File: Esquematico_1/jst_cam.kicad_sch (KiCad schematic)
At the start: 19 parts, among them J1 Screw_Terminal_01x04, J2 Screw_Terminal_01x03, J3 Screw_Terminal_01x06, J4 Screw_Terminal_01x08, J5 USB_C_Receptacle_USB2.0_14P, J6 Screw_Terminal_01x05, U5 USBLC6-2SC6

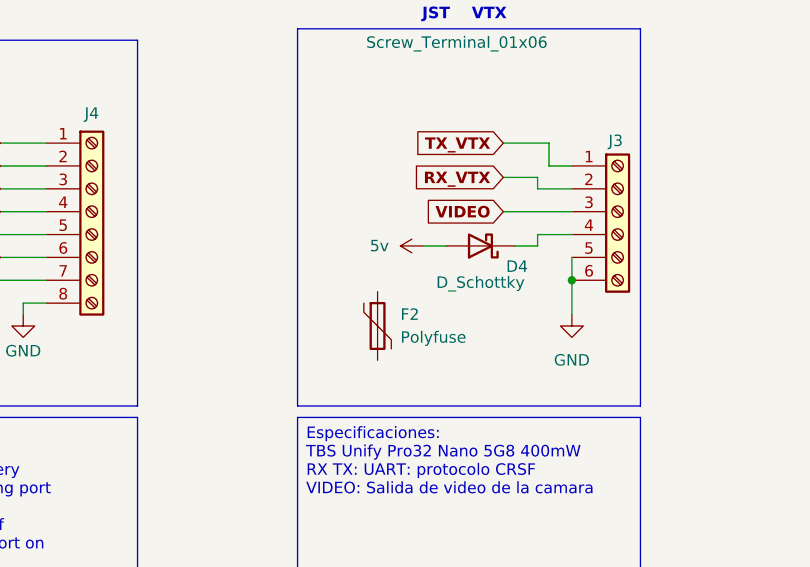
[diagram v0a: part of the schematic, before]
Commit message: Footprints
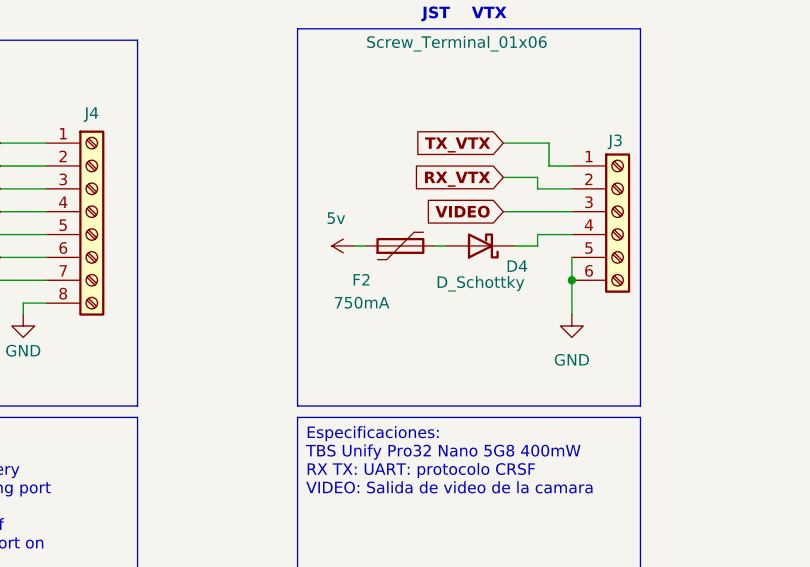
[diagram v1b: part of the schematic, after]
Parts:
- F2: value Polyfuse -> 750mA; footprint (none) -> Capacitor_SMD:C_0805_2012Metric_Pad1.18x1.45mm_HandSolder
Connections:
- net 5v: now also F2.1; no longer D4.2 (A)
- net at F2.2: now also D4.2 (A)
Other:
- moved on the sheet: F2
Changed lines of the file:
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@@
+	(wire
+		(pts
+			(xy 102.87 46.99) (xy 104.14 46.99)
+		)
+		(stroke
+			(width 0)
+			(type default)
+		)
+	)
 	(wire
 		(pts
@@
 	(wire
 		(pts
+			(xy 111.76 46.99) (xy 113.03 46.99)
+		)
+		(stroke
+			(width 0)
+			(type default)
+		)
+	)
+	(wire
+		(pts
 			(xy 144.78 128.27) (xy 154.94 128.27)
 		)
@@
 		(pts
 			(xy 119.38 39.37) (xy 123.19 39.37)
-		)
-		(stroke
-			(width 0)
-			(type default)
-		)
-	)
-	(wire
-		(pts
-			(xy 113.03 46.99) (xy 110.49 46.99)
 		)
 		(stroke
@@
 	(symbol
 		(lib_id "Device:Polyfuse")
-		(at 105.41 55.88 0)
+		(at 107.95 46.99 90)
 		(unit 1)
 		(exclude_from_sim no)
@@
 		(on_board yes)
 		(dnp no)
-		(fields_autoplaced yes)
 		(property "Reference" "F2"
-			(at 107.95 54.6099 0)
-			(effects
-				(font
-					(size 1.27 1.27)
-				)
-				(justify left)
-			)
-		)
-		(property "Value" "Polyfuse"
-			(at 107.95 57.1499 0)
-			(effects
-				(font
-					(size 1.27 1.27)
-				)
-				(justify left)
-			)
-		)
-		(property "Footprint" ""
-			(at 106.68 60.96 0)
+			(at 103.632 50.8 90)
+			(effects
+				(font
+					(size 1.27 1.27)
+				)
+			)
+		)
+		(property "Value" "750mA"
+			(at 103.632 53.34 90)
+			(effects
+				(font
+					(size 1.27 1.27)
+				)
+			)
+		)
+		(property "Footprint" "Capacitor_SMD:C_0805_2012Metric_Pad1.18x1.45mm_HandSolder"
+			(at 113.03 45.72 0)
 			(effects
 				(font
@@
 		)
 		(property "Datasheet" "~"
-			(at 105.41 55.88 0)
+			(at 107.95 46.99 0)
 			(effects
 				(font
@@
 		)
 		(property "Description" "Resettable fuse, polymeric positive temperature coefficient"
-			(at 105.41 55.88 0)
+			(at 107.95 46.99 0)
 			(effects
 				(font
@@
 	(symbol
 		(lib_id "power:+3.3V")
-		(at 110.49 46.99 90)
+		(at 102.87 46.99 90)
 		(unit 1)
 		(exclude_from_sim no)
@@
 		(on_board yes)
 		(dnp no)
-		(fields_autoplaced yes)
 		(property "Reference" "#PWR046"
-			(at 114.3 46.99 0)
+			(at 106.68 46.99 0)
 			(effects
 				(font
@@
 		)
 		(property "Value" "5v"
-			(at 106.68 46.9899 90)
+			(at 101.854 43.942 90)
 			(effects
 				(font
@@
 		)
 		(property "Footprint" ""
-			(at 110.49 46.99 0)
+			(at 102.87 46.99 0)
 			(effects
 				(font
@@
 		)
 		(property "Datasheet" ""
-			(at 110.49 46.99 0)
+			(at 102.87 46.99 0)
 			(effects
 				(font
@@
 		)
 		(property "Description" "Power symbol creates a global label with name \"+3.3V\""
-			(at 110.49 46.99 0)
-			(effects
-				(font
+			(at 102.87 46.99 0)
+			(effects
+				(font

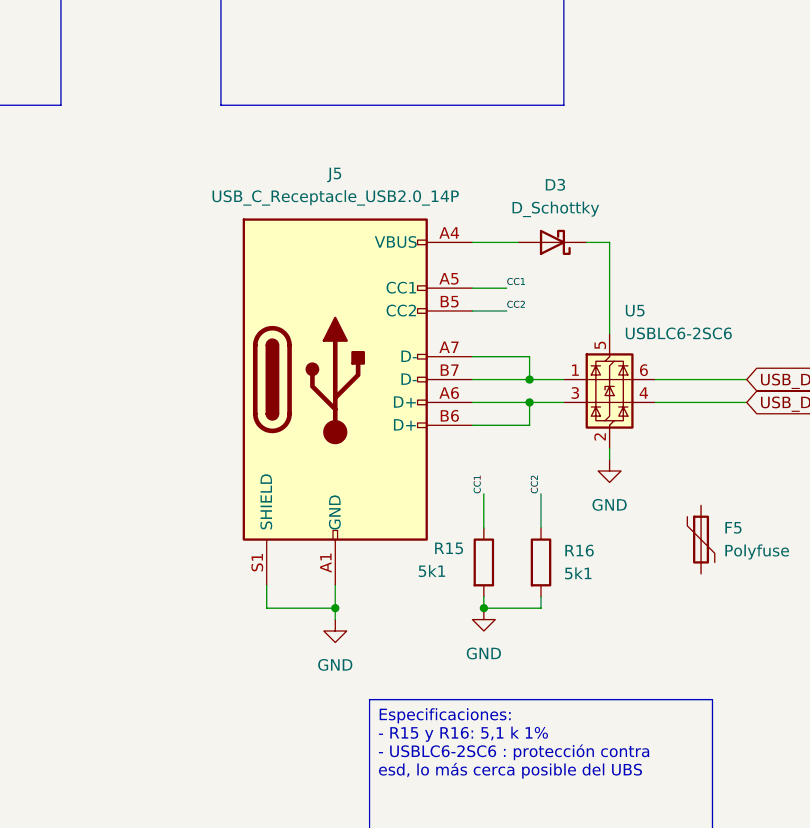
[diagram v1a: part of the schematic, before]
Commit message: USB 16 Pin
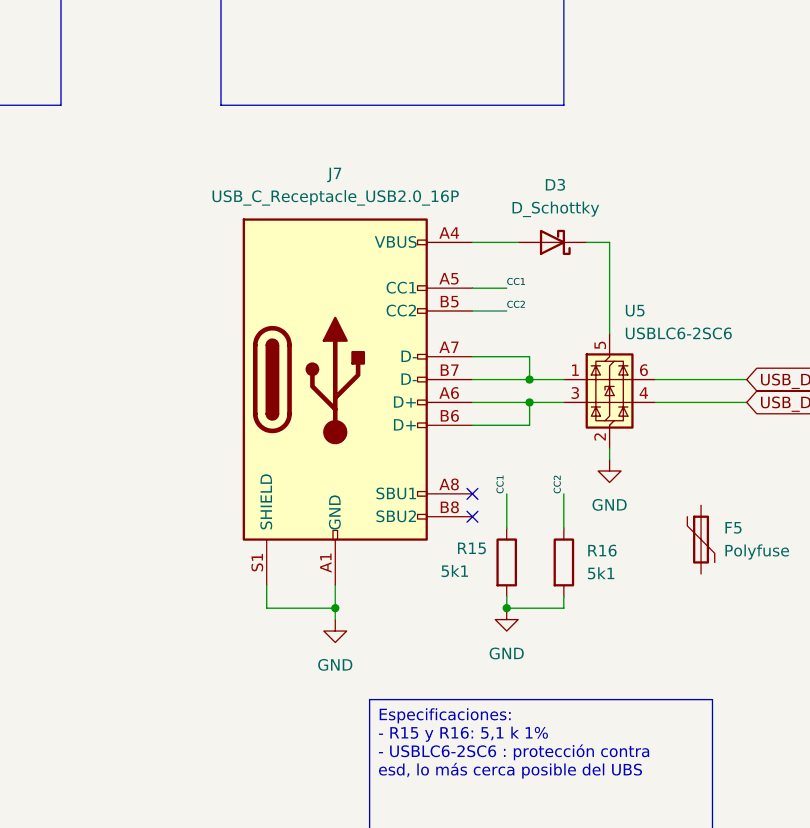
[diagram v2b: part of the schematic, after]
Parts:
- removed J5: USB_C_Receptacle_USB2.0_14P, symbol Connector:USB_C_Receptacle_USB2.0_14P
- added J7: USB_C_Receptacle_USB2.0_16P, symbol Connector:USB_C_Receptacle_USB2.0_16P
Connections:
- net CC1: now also J7.A5 (CC1)
- net CC2: now also J7.B5 (CC2)
- net GND: now also J7.A1 (GND), J7.A12 (GND), J7.B1 (GND), J7.B12 (GND), J7.S1 (SHIELD)
- net at D3.2 (A): now also J7.A4 (VBUS), J7.A9 (VBUS), J7.B4 (VBUS), J7.B9 (VBUS)
- net at U5.3 (I/O2): now also J7.A6 (D+), J7.B6 (D+)
- net at U5.1 (I/O1): now also J7.A7 (D-), J7.B7 (D-)
- no-connect marks 0 -> 2
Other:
- moved on the sheet: R15, R16
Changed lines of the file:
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@@
 	)
 	(junction
-		(at 125.73 153.67)
+		(at 128.27 153.67)
 		(diameter 0)
 		(color 0 0 0 0)
@@
 		(color 0 0 0 0)
 	)
+	(no_connect
+		(at 124.46 143.51)
+	)
+	(no_connect
+		(at 124.46 140.97)
+	)
 	(wire
 		(pts
@@
 	(wire
 		(pts
-			(xy 125.73 140.97) (xy 125.73 144.78)
+			(xy 128.27 140.97) (xy 128.27 144.78)
 		)
 		(stroke
@@
 	(wire
 		(pts
-			(xy 132.08 152.4) (xy 132.08 153.67)
+			(xy 134.62 152.4) (xy 134.62 153.67)
 		)
 		(stroke
@@
 	(wire
 		(pts
-			(xy 132.08 140.97) (xy 132.08 144.78)
+			(xy 134.62 140.97) (xy 134.62 144.78)
 		)
 		(stroke
@@
 	(wire
 		(pts
-			(xy 125.73 152.4) (xy 125.73 153.67)
+			(xy 128.27 152.4) (xy 128.27 153.67)
 		)
 		(stroke
@@
 	(wire
 		(pts
-			(xy 125.73 153.67) (xy 132.08 153.67)
+			(xy 128.27 153.67) (xy 134.62 153.67)
 		)
 		(stroke
@@
 	)
 	(label "CC1"
-		(at 125.73 140.97 90)
+		(at 128.27 140.97 90)
 		(effects
 			(font
@@
 	)
 	(label "CC2"
-		(at 132.08 140.97 90)
+		(at 134.62 140.97 90)
 		(effects
 			(font
@@
 	)
 	(symbol
-		(lib_id "Connector:USB_C_Receptacle_USB2.0_14P")
-		(at 109.22 128.27 0)
-		(unit 1)
-		(exclude_from_sim no)
-		(in_bom yes)
-		(on_board yes)
-		(dnp no)
-		(property "Reference" "J5"
-			(at 109.22 105.41 0)
-			(effects
-				(font
-					(size 1.27 1.27)
-				)
-			)
-		)
-		(property "Value" "USB_C_Receptacle_USB2.0_14P"
-			(at 109.22 107.95 0)
-			(effects
-				(font
-					(size 1.27 1.27)
-				)
-			)
-		)
-		(property "Footprint" ""
-			(at 113.03 128.27 0)
-			(effects
-				(font
-					(size 1.27 1.27)
-				)
-				(hide yes)
-			)
-		)
-		(property "Datasheet" "https://www.usb.org/sites/default/files/documents/usb_type-c.zip"
-			(at 113.03 128.27 0)
-			(effects
-				(font
-					(size 1.27 1.27)
-				)
-				(hide yes)
-			)
-		)
-		(property "Description" "USB 2.0-only 14P Type-C Receptacle connector"
-			(at 109.22 128.27 0)
-			(effects
-				(font
-					(size 1.27 1.27)
-				)
-				(hide yes)
-			)
-		)
-		(pin "B7"
-		)
-		(pin "B5"
-		)
-		(pin "B6"
-		)
-		(pin "A6"
-		)
-		(pin "B4"
-		)
-		(pin "A7"
-		)
-		(pin "S1"
-		)
-		(pin "B9"
-		)
-		(pin "A5"
-		)
-		(pin "A1"
-		)
-		(pin "A12"
-		)
-		(pin "B1"
-		)
-		(pin "B12"
-		)
-		(pin "A4"
-		)
-		(pin "A9"
-		)
-		(instances
-			(project "Esquematico_1"
-				(path "/de2d80c1-c21c-478d-b724-17659b714c38/457e76de-adfe-4ec5-a818-c5970caa89a7"
-					(reference "J5")
-					(unit 1)
-				)
-			)
-		)
-	)
-	(symbol
 		(lib_id "power:GND")
 		(at 66.04 54.61 0)
@@
 	)
 	(symbol
+		(lib_id "Connector:USB_C_Receptacle_USB2.0_16P")
+		(at 109.22 128.27 0)
+		(unit 1)
+		(exclude_from_sim no)
+		(in_bom yes)
+		(on_board yes)
+		(dnp no)
+		(fields_autoplaced yes)
+		(property "Reference" "J7"
+			(at 109.22 105.41 0)
+			(effects
+				(font
+					(size 1.27 1.27)
+				)
+			)
+		)
+		(property "Value" "USB_C_Receptacle_USB2.0_16P"
+			(at 109.22 107.95 0)
+			(effects
+				(font
+					(size 1.27 1.27)
+				)
+			)
+		)
+		(property "Footprint" ""
+			(at 113.03 128.27 0)
+			(effects
+				(font
+					(size 1.27 1.27)
+				)
+				(hide yes)
+			)
+		)
+		(property "Datasheet" "https://www.usb.org/sites/default/files/documents/usb_type-c.zip"
+			(at 113.03 128.27 0)
+			(effects
+				(font
+					(size 1.27 1.27)
+				)
+				(hide yes)
+			)
+		)
+		(property "Description" "USB 2.0-only 16P Type-C Receptacle connector"
+			(at 109.22 128.27 0)
+			(effects
+				(font
+					(size 1.27 1.27)
+				)
+				(hide yes)
+			)
+		)
+		(pin "B6"
+		)
+		(pin "B4"
+		)
+		(pin "A7"
+		)
+		(pin "A5"
+		)
+		(pin "A1"
+		)
+		(pin "A12"
+		)
+		(pin "A9"
+		)
+		(pin "S1"
+		)
+		(pin "A4"
+		)
+		(pin "B12"
+		)
+		(pin "B1"
+		)
+		(pin "B7"
+		)
+		(pin "A6"
+		)
+		(pin "B9"
+		)
+		(pin "B8"
+		)
+		(pin "B5"
+		)
+		(pin "A8"
+		)
+		(instances
+			(project ""
+				(path "/de2d80c1-c21c-478d-b724-17659b714c38/457e76de-adfe-4ec5-a818-c5970caa89a7"
+					(reference "J7")
+					(unit 1)
+				)
+			)
+		)
+	)
+	(symbol
 		(lib_id "Device:D_Schottky")
 		(at 133.35 113.03 180)
@@
 	(symbol
 		(lib_id "Device:R")
-		(at 132.08 148.59 0)
+		(at 134.62 148.59 0)
 		(unit 1)
 		(exclude_from_sim no)
@@
 		(fields_autoplaced yes)
 		(property "Reference" "R16"
-			(at 134.62 147.3199 0)
+			(at 137.16 147.3199 0)
 			(effects
 				(font
@@
 		)
 		(property "Value" "5k1"
-			(at 134.62 149.8599 0)
+			(at 137.16 149.8599 0)
 			(effects
 				(font
@@
 		)
 		(property "Footprint" "Resistor_SMD:R_0805_2012Metric_Pad1.20x1.40mm_HandSolder"
-			(at 130.302 148.59 90)
+			(at 132.842 148.59 90)
 			(effects
 				(font
@@
 		)
 		(property "Datasheet" "~"
-			(at 132.08 148.59 0)
+			(at 134.62 148.59 0)
 			(effects
 				(font
@@
 		)
 		(property "Description" "Resistor"
-			(at 132.08 148.59 0)
+			(at 134.62 148.59 0)
 			(effects
 				(font
@@
 	(symbol
 		(lib_id "power:GND")
-		(at 125.73 153.67 0)
+		(at 128.27 153.67 0)
 		(unit 1)
 		(exclude_from_sim no)
@@
 		(fields_autoplaced yes)
 		(property "Reference" "#PWR043"
-			(at 125.73 160.02 0)
+			(at 128.27 160.02 0)
 			(effects
 				(font
@@
 		)
 		(property "Value" "GND"
-			(at 125.73 158.75 0)
+			(at 128.27 158.75 0)
 			(effects
 				(font
@@
 		)
 		(property "Footprint" ""
-			(at 125.73 153.67 0)
+			(at 128.27 153.67 0)
 			(effects
 				(font
@@
 		)
 		(property "Datasheet" ""
-			(at 125.73 153.67 0)
+			(at 128.27 153.67 0)
 			(effects
 				(font
@@
 		)
 		(property "Description" "Power symbol creates a global label with name \"GND\" , ground"
-			(at 125.73 153.67 0)
+			(at 128.27 153.67 0)
 			(effects
 				(font
@@
 	(symbol
 		(lib_id "Device:R")
-		(at 125.73 148.59 0)
+		(at 128.27 148.59 0)
 		(unit 1)
 		(exclude_from_sim no)
@@
 		(dnp no)
 		(property "Reference" "R15"
-			(at 120.142 147.066 0)
+			(at 122.682 147.066 0)
 			(effects
 				(font
@@
 		)
 		(property "Value" "5k1"
-			(at 118.364 149.606 0)
+			(at 120.904 149.606 0)
 			(effects
 				(font
@@
 		)
 		(property "Footprint" "Resistor_SMD:R_0805_2012Metric_Pad1.20x1.40mm_HandSolder"
-			(at 123.952 148.59 90)
+			(at 126.492 148.59 90)
 			(effects
 				(font
@@
 		)
 		(property "Datasheet" "~"
-			(at 125.73 148.59 0)
+			(at 128.27 148.59 0)
 			(effects
 				(font
@@
 		)
 		(property "Description" "Resistor"
-			(at 125.73 148.59 0)
+			(at 128.27 148.59 0)
 			(effects
 				(font
